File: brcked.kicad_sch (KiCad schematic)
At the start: 6 parts, among them J1 INMP441, J2 MAX98-, J3 screen, J4 raspberry_pi_0, J5 battery, J6 IP5306

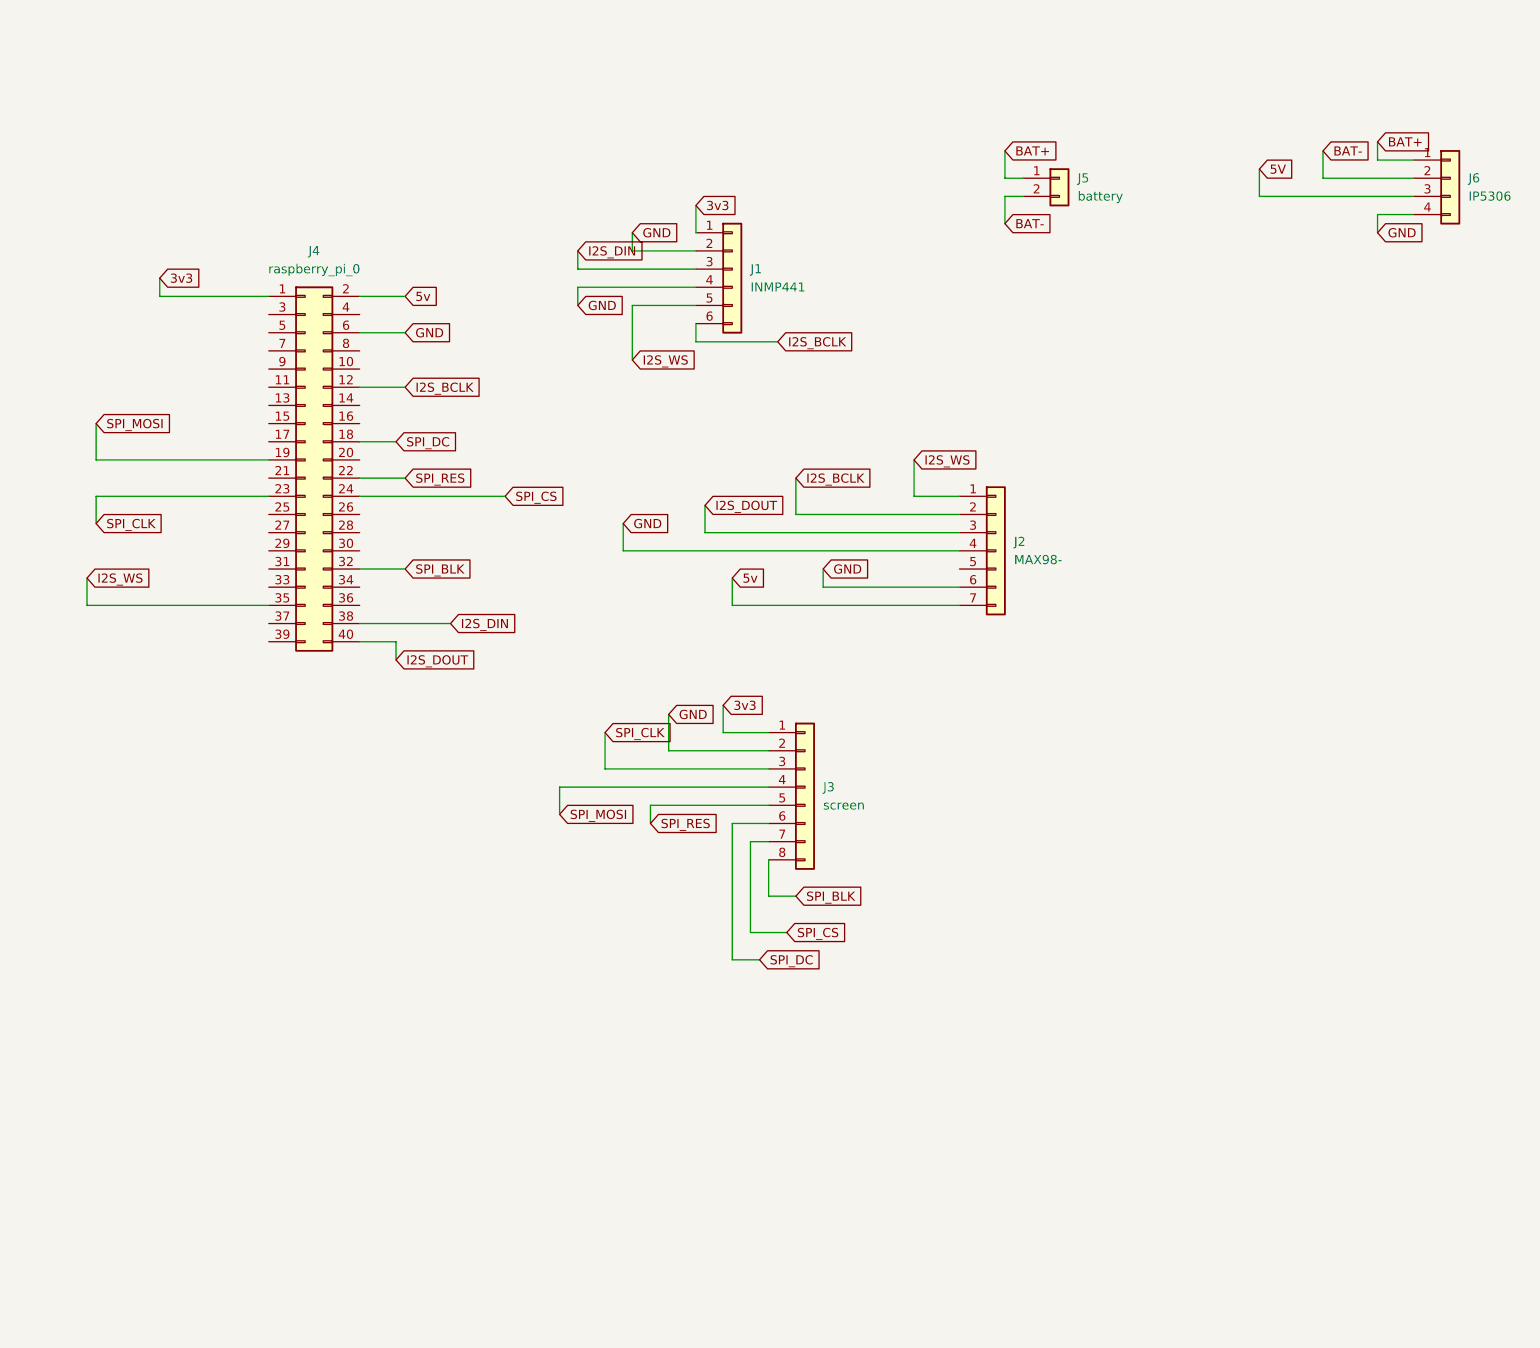
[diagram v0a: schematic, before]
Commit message: completed the schematic and checked it like 10 times
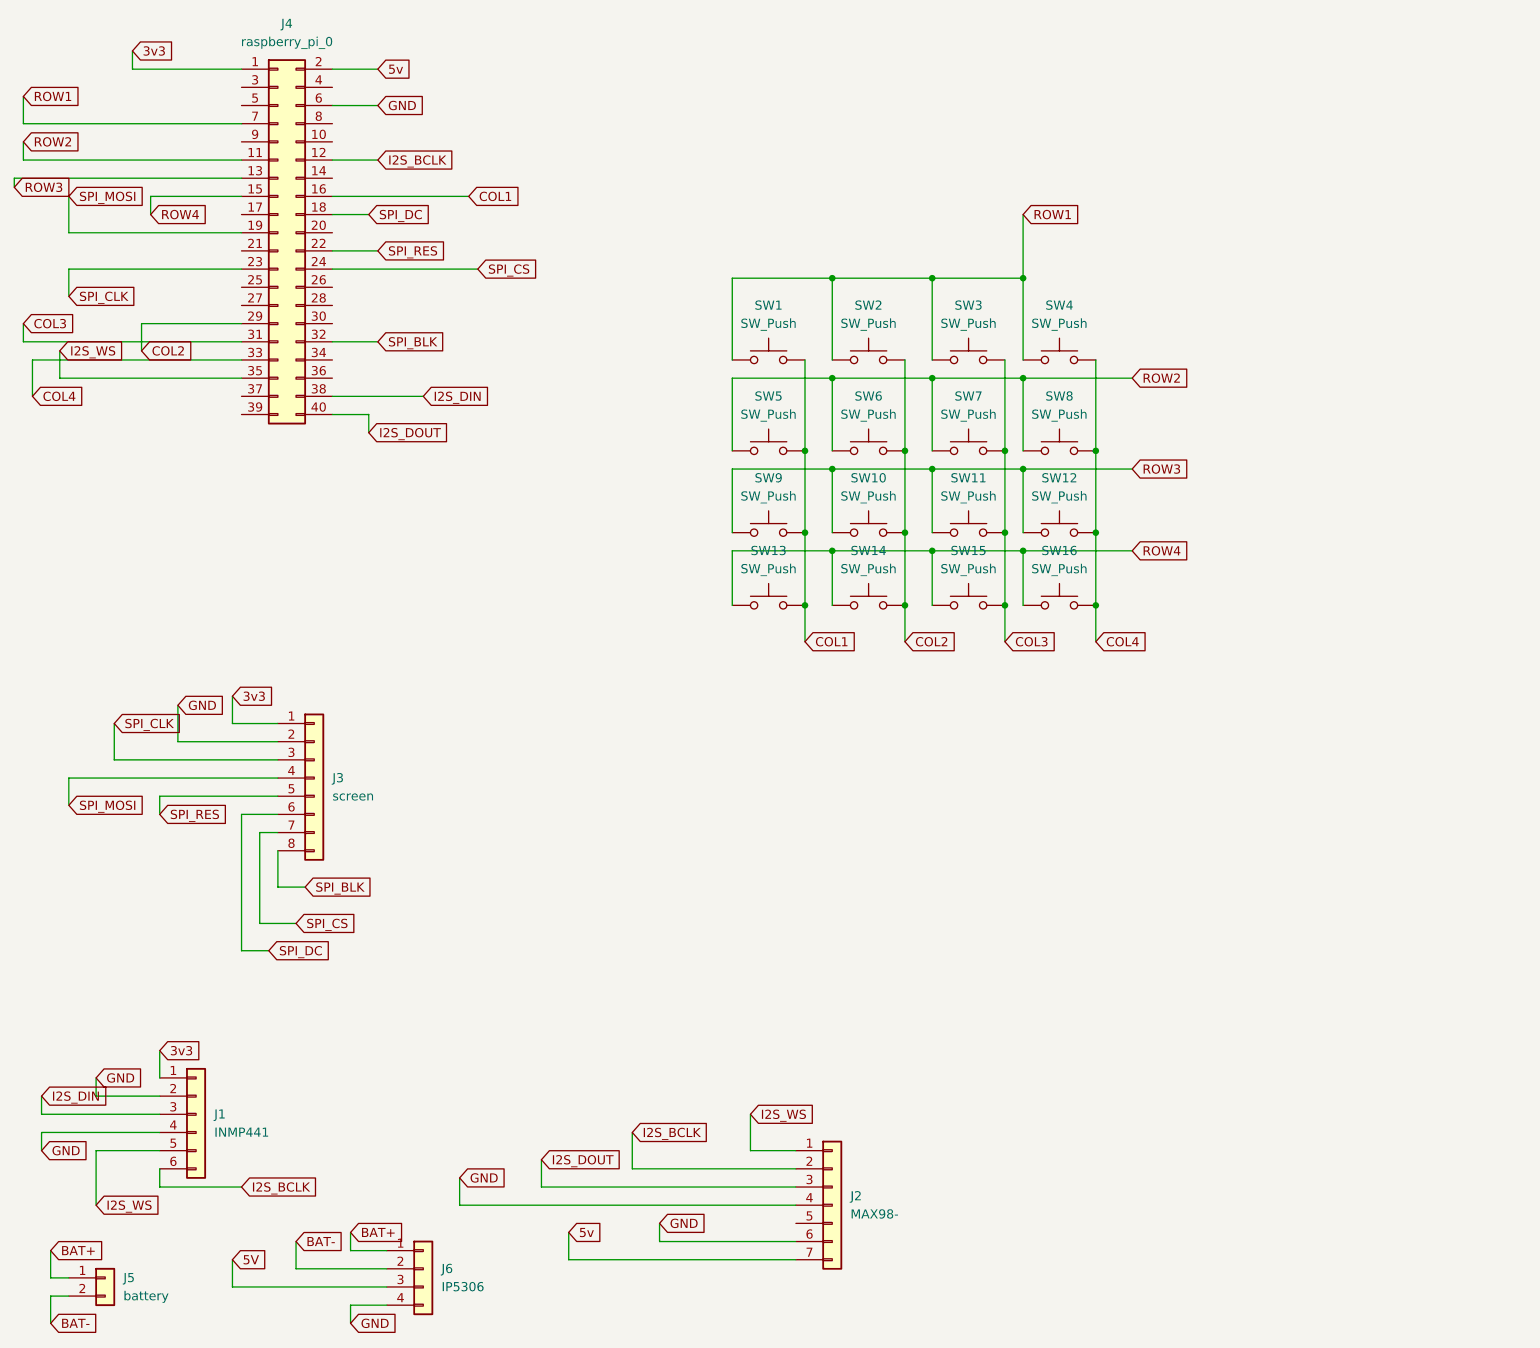
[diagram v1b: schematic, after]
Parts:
- added SW1: SW_Push, Button_Switch_THT:SW_NKK_GW12LJP, symbol Switch:SW_Push
- added SW10, SW11, SW12, SW13, SW14, SW15, SW16, SW2, SW3, SW4, SW5, SW6, SW7, SW8, SW9: SW_Push, symbol Switch:SW_Push
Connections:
- net ROW2: now reaches J4.11 (Pin_11)
- net ROW2: now also SW5.1, SW6.1, SW7.1, SW8.1
- net ROW3: now reaches J4.13 (Pin_13)
- net ROW3: now also SW10.1, SW11.1, SW12.1, SW9.1
- net ROW4: now reaches J4.15 (Pin_15)
- net ROW4: now also SW13.1, SW14.1, SW15.1, SW16.1
- net COL1: now reaches J4.16 (Pin_16)
- net COL1: now also SW1.2, SW13.2, SW5.2, SW9.2
- net COL2: now reaches J4.29 (Pin_29)
- net COL2: now also SW10.2, SW14.2, SW2.2, SW6.2
- net COL3: now reaches J4.31 (Pin_31)
- net COL3: now also SW11.2, SW15.2, SW3.2, SW7.2
- net COL4: now reaches J4.33 (Pin_33)
- net COL4: now also SW12.2, SW16.2, SW4.2, SW8.2
- net ROW1: now reaches J4.7 (Pin_7)
- net ROW1: now also SW1.1, SW2.1, SW3.1, SW4.1
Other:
- moved on the sheet: J1, J2, J3, J4, J5, J6

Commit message: finished pcb and routing, 3d model's next
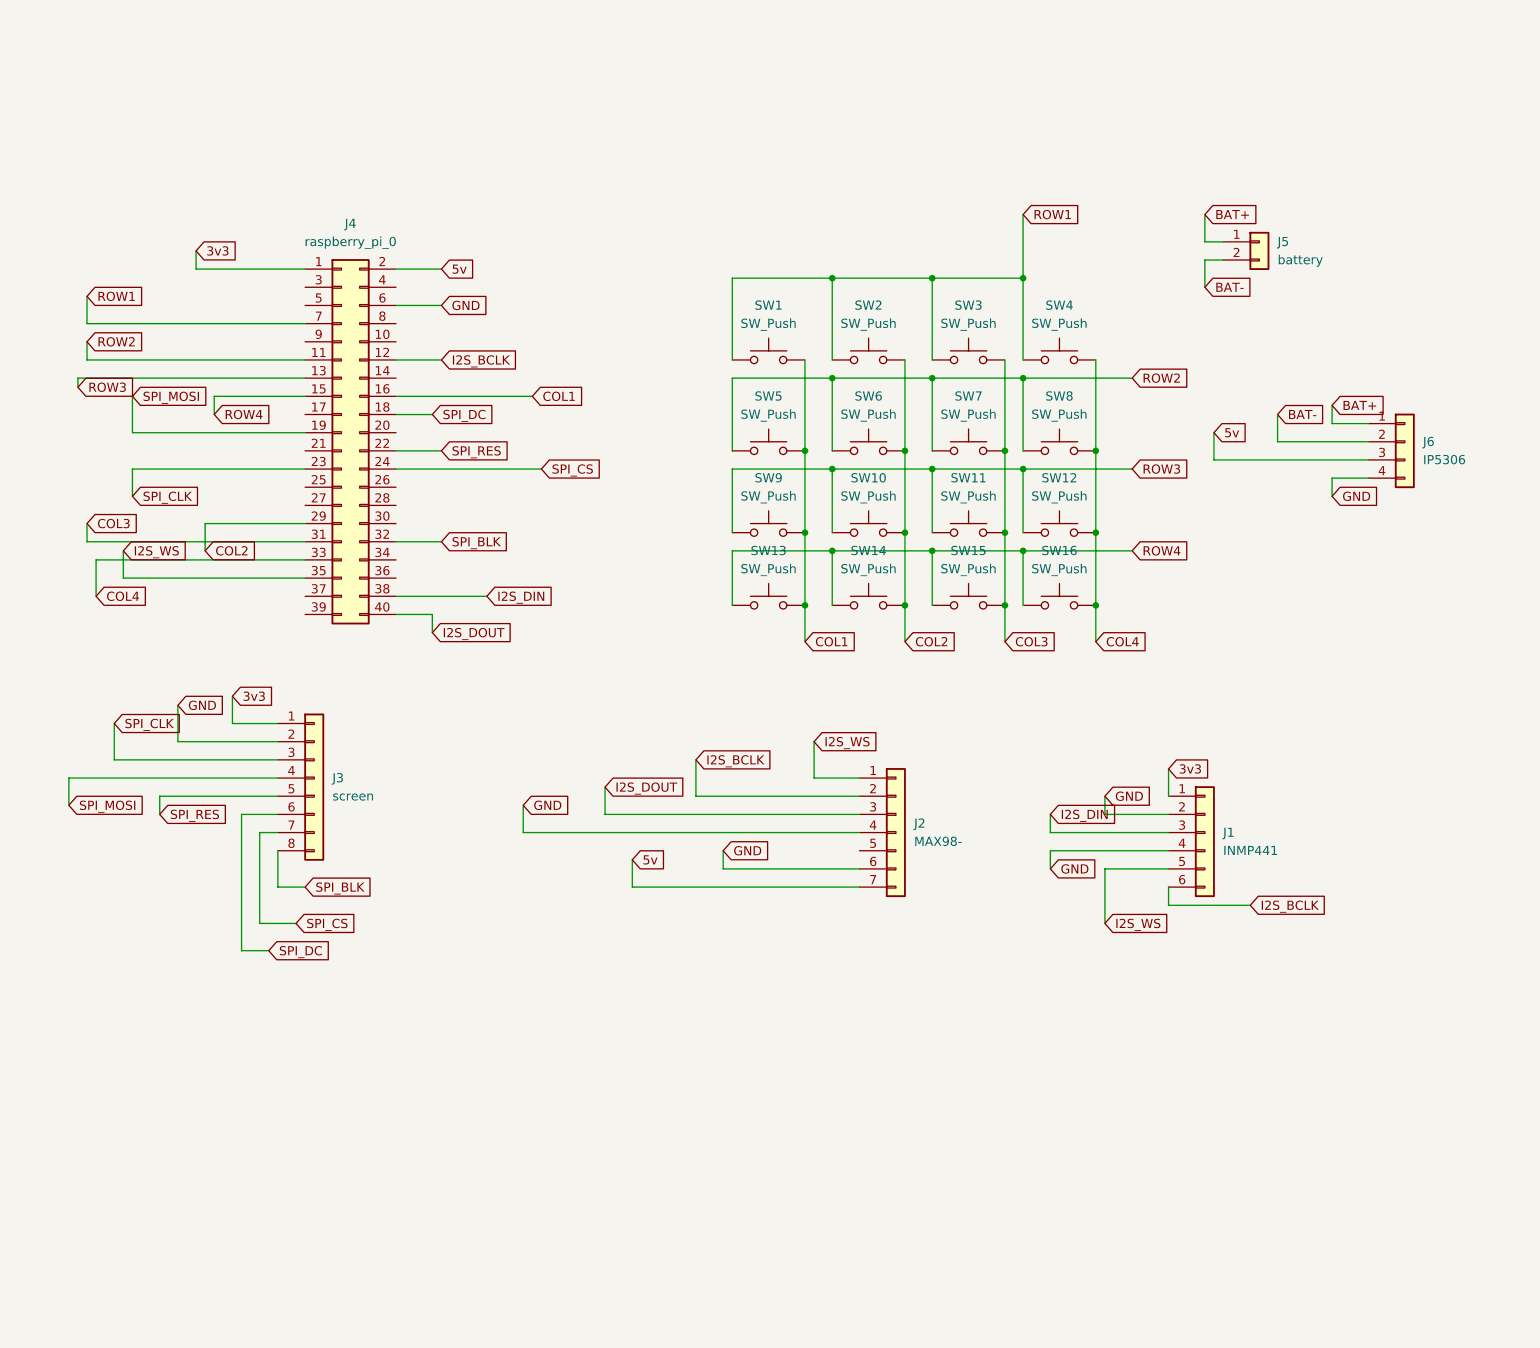
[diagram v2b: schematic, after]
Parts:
- J1: footprint Module:RaspberryPi_Pico_SMD -> Connector_PinHeader_2.54mm:PinHeader_1x06_P2.54mm_Vertical
- J2: footprint (none) -> Connector_PinHeader_2.54mm:PinHeader_1x07_P2.54mm_Vertical
- J3: footprint (none) -> Connector_PinHeader_2.54mm:PinHeader_1x08_P2.54mm_Vertical
- J4: footprint Module:RaspberryPi_Pico_Common_Unspecified -> Connector_PinHeader_2.54mm:PinHeader_2x20_P2.54mm_Vertical
- J5: footprint (none) -> Connector_PinHeader_2.54mm:PinHeader_1x02_P2.54mm_Vertical
- J6: footprint (none) -> Connector_PinHeader_2.54mm:PinHeader_1x04_P2.54mm_Vertical
- SW1: footprint Button_Switch_THT:SW_NKK_GW12LJP -> Button_Switch_THT:SW_PUSH_6mm
- SW10, SW11, SW12, SW13, SW14, SW15, SW16, SW2, SW3, SW4, SW5, SW6, SW7, SW8, SW9: footprint (none) -> Button_Switch_THT:SW_PUSH_6mm
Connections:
- net 5V is gone; now on net 5v: J6.3 (Pin_3)
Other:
- moved on the sheet: J1, J2, J4, J5, J6
